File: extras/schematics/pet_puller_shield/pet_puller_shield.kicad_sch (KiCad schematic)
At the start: 19 parts, among them J1 Jack-DC, J2 Conn_01x02, J3 Conn_01x02, J4 Conn_01x02, J5 Conn_01x04, Q1 IRF540N, U1 LM317_TO-220, U2 MX1508_module

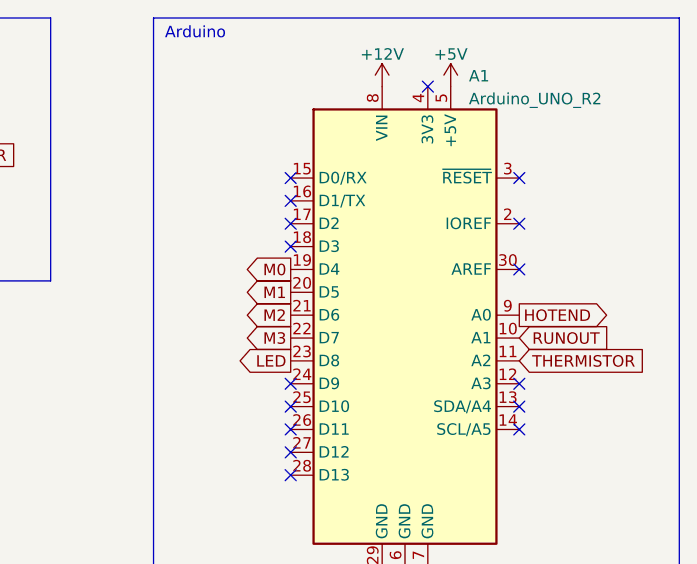
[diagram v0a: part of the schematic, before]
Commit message: Update schematics
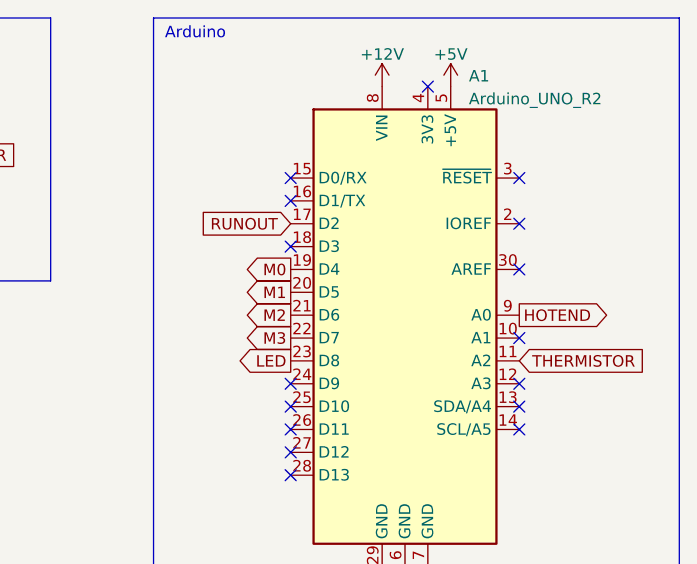
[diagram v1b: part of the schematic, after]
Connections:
- net RUNOUT: now also A1.17 (D2); no longer A1.10 (A1)
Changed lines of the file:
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@@
   (no_connect (at 252.73 39.37))
   (no_connect (at 252.73 44.45))
-  (no_connect (at 227.33 39.37))
   (no_connect (at 227.33 67.31))
   (no_connect (at 242.57 24.13))
+  (no_connect (at 252.73 52.07))
   (no_connect (at 252.73 59.69))
   (no_connect (at 227.33 59.69))
@@
     (effects (font (size 1.27 1.27)) (justify left bottom))
   )
-  (global_label "RUNOUT" (shape input) (at 252.73 52.07 0) (fields_autoplaced)
-    (effects (font (size 1.27 1.27)) (justify left))
-    (property "Intersheet References" "${INTERSHEET_REFS}" (id 0) (at 262.7026 52.1494 0)
-      (effects (font (size 1.27 1.27)) (justify left) hide)
-    )
-  )
   (global_label "M3" (shape output) (at 227.33 52.07 180) (fields_autoplaced)
     (effects (font (size 1.27 1.27)) (justify right))
@@
     )
   )
+  (global_label "RUNOUT" (shape input) (at 227.33 39.37 180) (fields_autoplaced)
+    (effects (font (size 1.27 1.27)) (justify right))
+    (property "Intersheet References" "${INTERSHEET_REFS}" (id 0) (at 217.3574 39.2906 0)
+      (effects (font (size 1.27 1.27)) (justify right) hide)
+    )
+  )

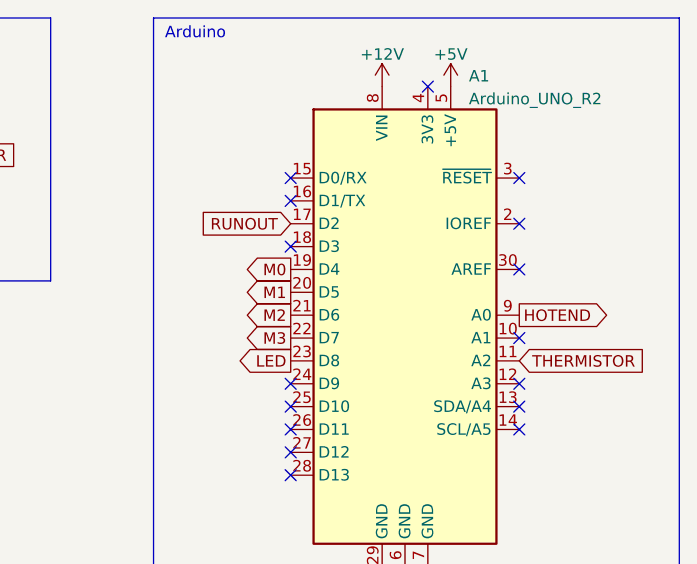
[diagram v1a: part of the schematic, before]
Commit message: Update schematics
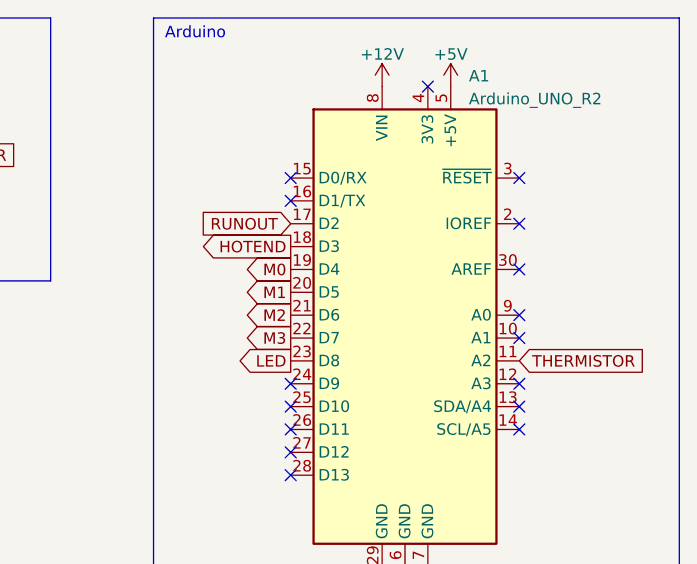
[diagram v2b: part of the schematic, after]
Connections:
- net HOTEND: now also A1.18 (D3); no longer A1.9 (A0)
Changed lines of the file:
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@@
   (no_connect (at 252.73 44.45))
   (no_connect (at 227.33 67.31))
+  (no_connect (at 252.73 49.53))
   (no_connect (at 242.57 24.13))
   (no_connect (at 252.73 52.07))
@@
   (no_connect (at 227.33 62.23))
   (no_connect (at 252.73 62.23))
-  (no_connect (at 227.33 41.91))
   (wire (pts (xy 44.45 54.61) (xy 44.45 59.69))
     (stroke (width 0) (type default) (color 0 0 0 0))
@@
     )
   )
-  (global_label "HOTEND" (shape output) (at 252.73 49.53 0) (fields_autoplaced)
-    (effects (font (size 1.27 1.27)) (justify left))
-    (property "Intersheet References" "${INTERSHEET_REFS}" (id 0) (at 262.5212 49.6094 0)
-      (effects (font (size 1.27 1.27)) (justify left) hide)
-    )
-  )
+  (global_label "HOTEND" (shape output) (at 227.33 41.91 180) (fields_autoplaced)
+    (effects (font (size 1.27 1.27)) (justify right))
+    (property "Intersheet References" "${INTERSHEET_REFS}" (id 0) (at 217.5388 41.8306 0)
+      (effects (font (size 1.27 1.27)) (justify right) hide)
+    )
+  )
